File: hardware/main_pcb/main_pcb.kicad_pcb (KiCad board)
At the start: 4 copper layers, 44.5 x 44.5 mm, 57 parts, among them J1 USB_C_Receptacle_USB2.0, J2 Conn_01x03, J3 Conn_01x14, J4 Conn_01x14, J6 PROG, Q1 AO3400A, Q2 AO3400A, Q3 AO3400A, SW1 SW_SPST, U1 IP5306, U2 SN74LVC1T45DCK, U3 AP63200WU, U4 ESP32-S3-WROOM-1U-N8R2

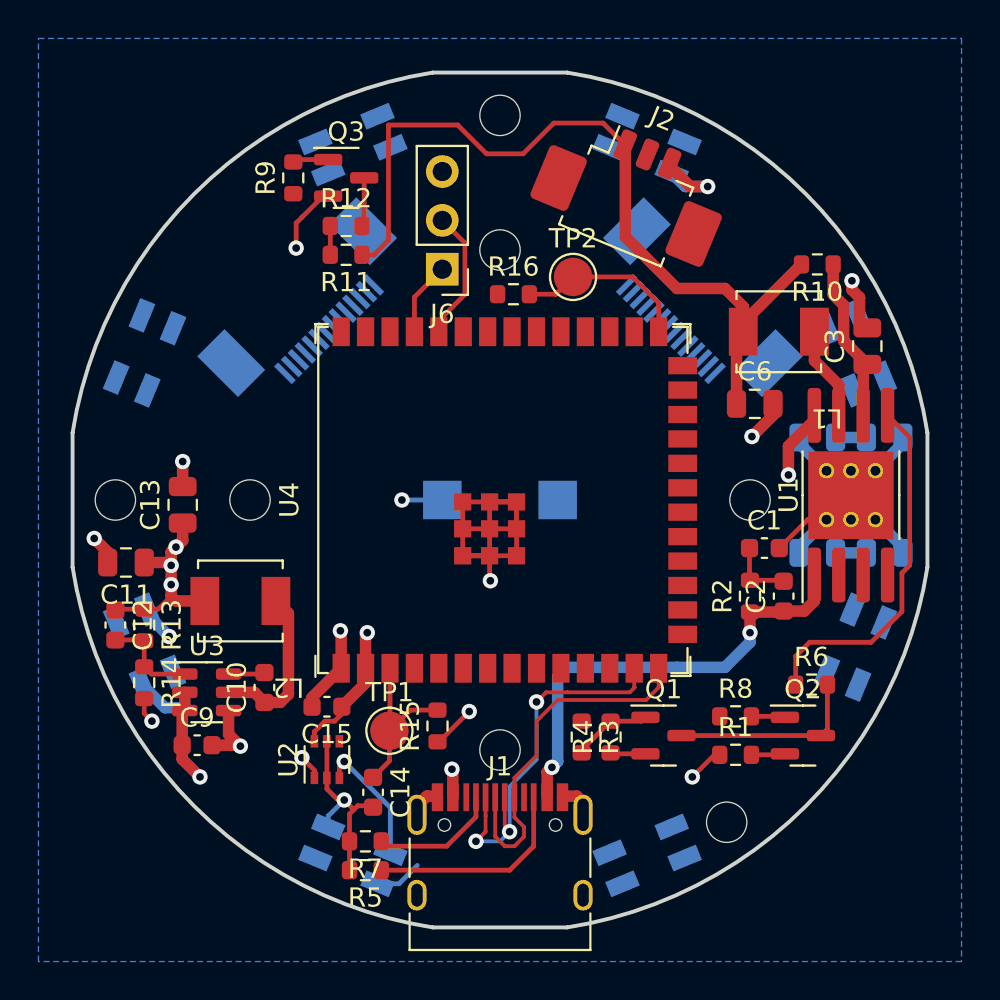
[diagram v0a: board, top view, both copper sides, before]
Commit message: Finished routing
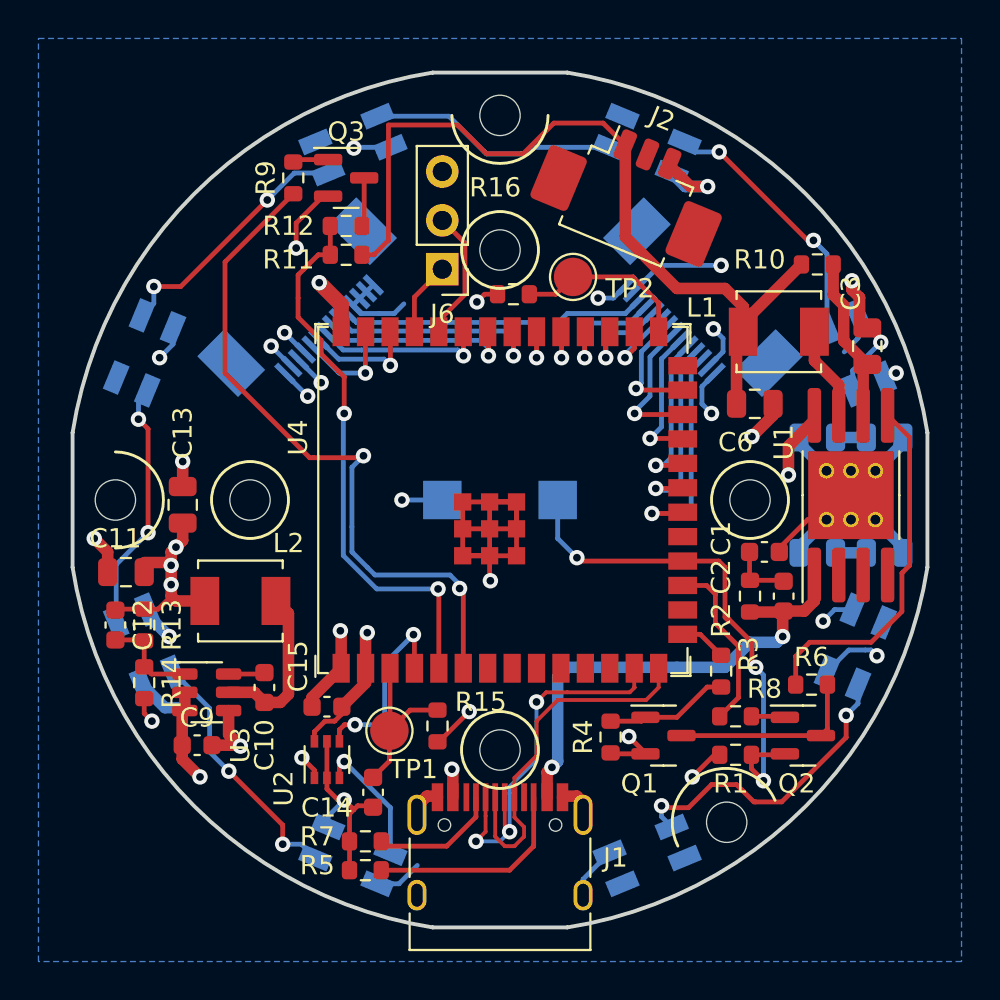
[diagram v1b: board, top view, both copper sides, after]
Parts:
- moved R3 8.02 mm to (61.5, 58.9)
- moved C11 0.50 mm to (30.6, 53.8)
- moved C1 0.20 mm to (63.8, 52.7)
- turned D6 to -157.5 degrees
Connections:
- U4 pad 15: unconnected-(U4-Pad15) -> IO_OFF
- U4 pad 17: unconnected-(U4-Pad17) -> PUSH_UP
- U4 pad 18: unconnected-(U4-Pad18) -> PUSH
- U4 pad 20: unconnected-(U4-Pad20) -> MOTOR_UH
- U4 pad 21: unconnected-(U4-Pad21) -> MOTOR_UL
- U4 pad 22: unconnected-(U4-Pad22) -> MOTOR_VH
- U4 pad 23: unconnected-(U4-Pad23) -> MOTOR_VL
- U4 pad 24: unconnected-(U4-Pad24) -> MOTOR_WH
- U4 pad 25: unconnected-(U4-Pad25) -> MOTOR_WL
- U4 pad 28: unconnected-(U4-Pad28) -> MOTOR_DIAG
- U4 pad 29: unconnected-(U4-Pad29) -> MM_SDA
- U4 pad 30: unconnected-(U4-Pad30) -> MM_SCL
- U4 pad 31: unconnected-(U4-Pad31) -> MM_CS
- U4 pad 32: unconnected-(U4-Pad32) -> LCD_BL
- U4 pad 33: unconnected-(U4-Pad33) -> LCD_DC
- U4 pad 34: unconnected-(U4-Pad34) -> LCD_CS
- U4 pad 35: unconnected-(U4-Pad35) -> LCD_SCL
- U4 pad 38: unconnected-(U4-Pad38) -> LCD_SDA
- U4 pad 39: unconnected-(U4-Pad39) -> LCD_RESET
- U4 pad 4: unconnected-(U4-Pad4) -> RGB
- U4 pad 5: unconnected-(U4-Pad5) -> BAT_ADC
- U4 pad 6: unconnected-(U4-Pad6) -> BAT_ADC_EN
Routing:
- net BAT_ADC_EN: track 0.00 -> 35.8 mm, vias 0 -> 2
- net GND: track 80.1 -> 111.5 mm, vias 13 -> 25
- net BAT_ADC: track 1.50 -> 29.0 mm, vias 0 -> 2
- net PUSH: track 1.76 -> 26.7 mm, vias 0 -> 3
- net Net-(D4-Pad3): track 0.00 -> 18.9 mm, vias 0 -> 2
- net Net-(D4-Pad1): track 0.00 -> 16.2 mm, vias 0 -> 2
- net Net-(D3-Pad1): track 0.00 -> 13.7 mm, vias 0 -> 2
- net Net-(D1-Pad1): track 0.00 -> 13.3 mm, vias 0 -> 2
- net Net-(D2-Pad1): track 0.00 -> 13.3 mm, vias 0 -> 2
- net Net-(D2-Pad3): track 0.00 -> 13.2 mm, vias 0 -> 2
- net LCD_BL: track 0.00 -> 13.1 mm, vias 0 -> 1
- net Net-(D3-Pad3): track 0.00 -> 13.0 mm
- net LCD_DC: track 0.00 -> 11.7 mm, vias 0 -> 1
- net MOTOR_UH: track 0.00 -> 11.6 mm, vias 0 -> 1
- net LCD_CS: track 0.00 -> 10.3 mm, vias 0 -> 1
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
